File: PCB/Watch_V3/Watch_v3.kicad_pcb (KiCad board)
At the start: 2 copper layers, 39 x 42.8 mm, 79 parts, among them J1 USB_C_Receptacle_USB2.0_16P, J2 Screw_Terminal, J4 OLED, J5 BN220, J7 MAX30102, J8 Conn_01x07_Pin, M1 Motor_DC, Q1 AO3401A, Q4 SI2302, Q5 BC847, SW1 SW_DPST_x2, SW2 SW_SPDT, SW3 SW_DPST_x2, SW4 Mode, SW5 Down, SW6 Select, SW7 Up, U1 AP2112K-3.3, U2 AP2112K-3.3, U3 TP4056, U4 ESP32-WROOM-32D, U6 MPU-6050

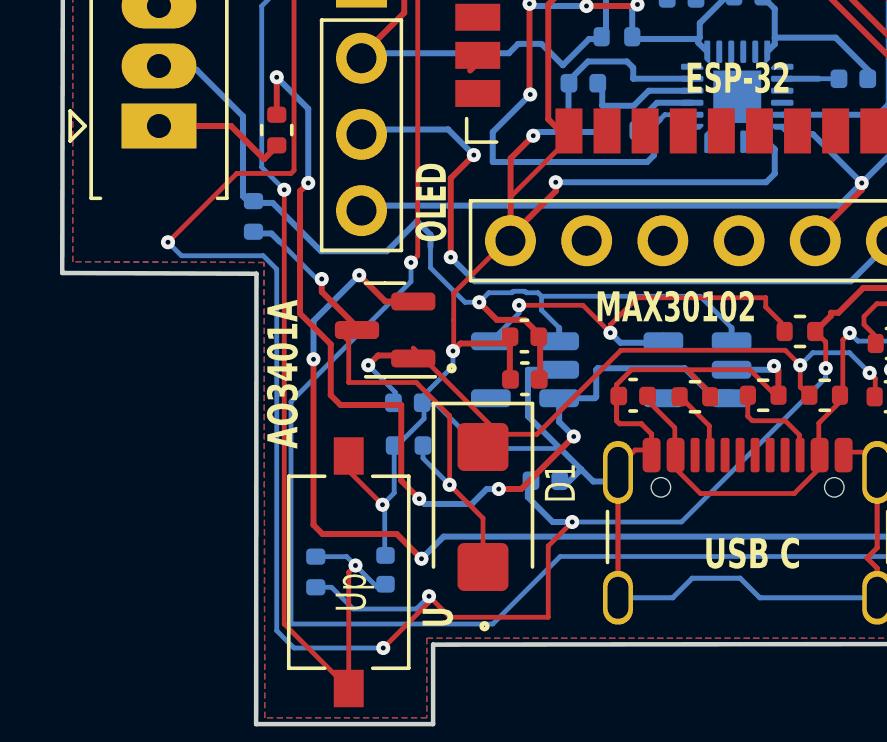
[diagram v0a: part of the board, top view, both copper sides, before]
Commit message: updating PCB design
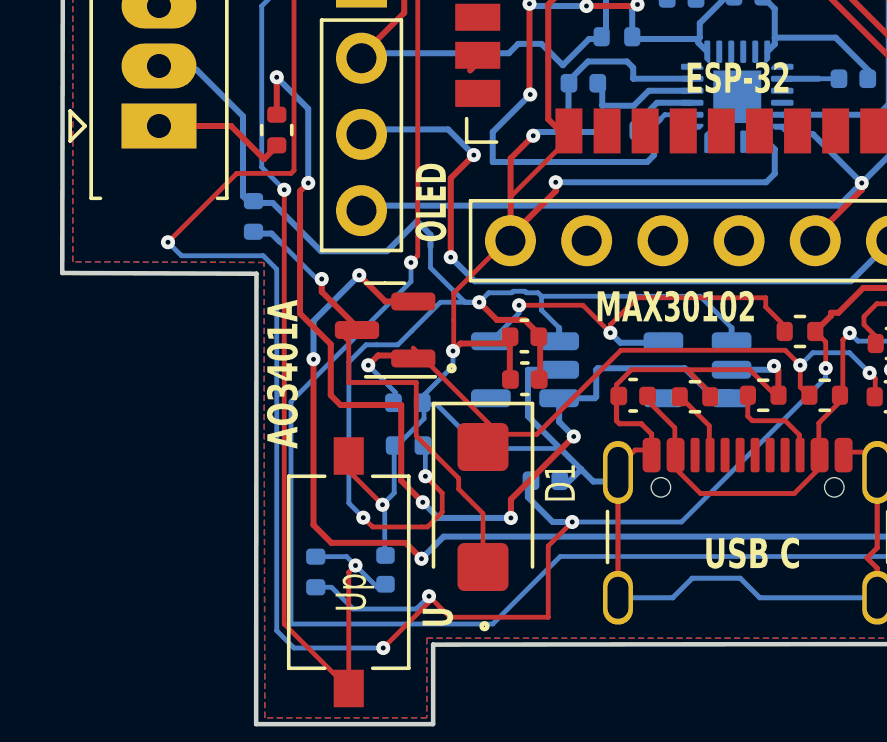
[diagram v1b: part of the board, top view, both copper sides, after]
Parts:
- R14: value 1K -> 10K
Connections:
- C2 pad 2: Net-(Q1-D) -> VBUS
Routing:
- net VBUS: track 32.7 -> 48.8 mm, vias 1 -> 3
- net Net-(Q1-D): track 17.5 -> 15.9 mm, vias 2 -> 1
- net ENA: track 34.0 -> 34.8 mm
